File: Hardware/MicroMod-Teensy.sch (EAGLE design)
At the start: 73 parts, among them J1 MICROMOD-2222, Q1 20V/4.2A/52mΩ/1.4W, Q2 20V/0.2A/8MHz/1.2Ω/1Vth, U1 IMXRT1062DV10X10, U3 MKL02Z32VFG4, U4 W25QXX128MBIT-6X5, Y1 32.768kHz, Y2 24MHz

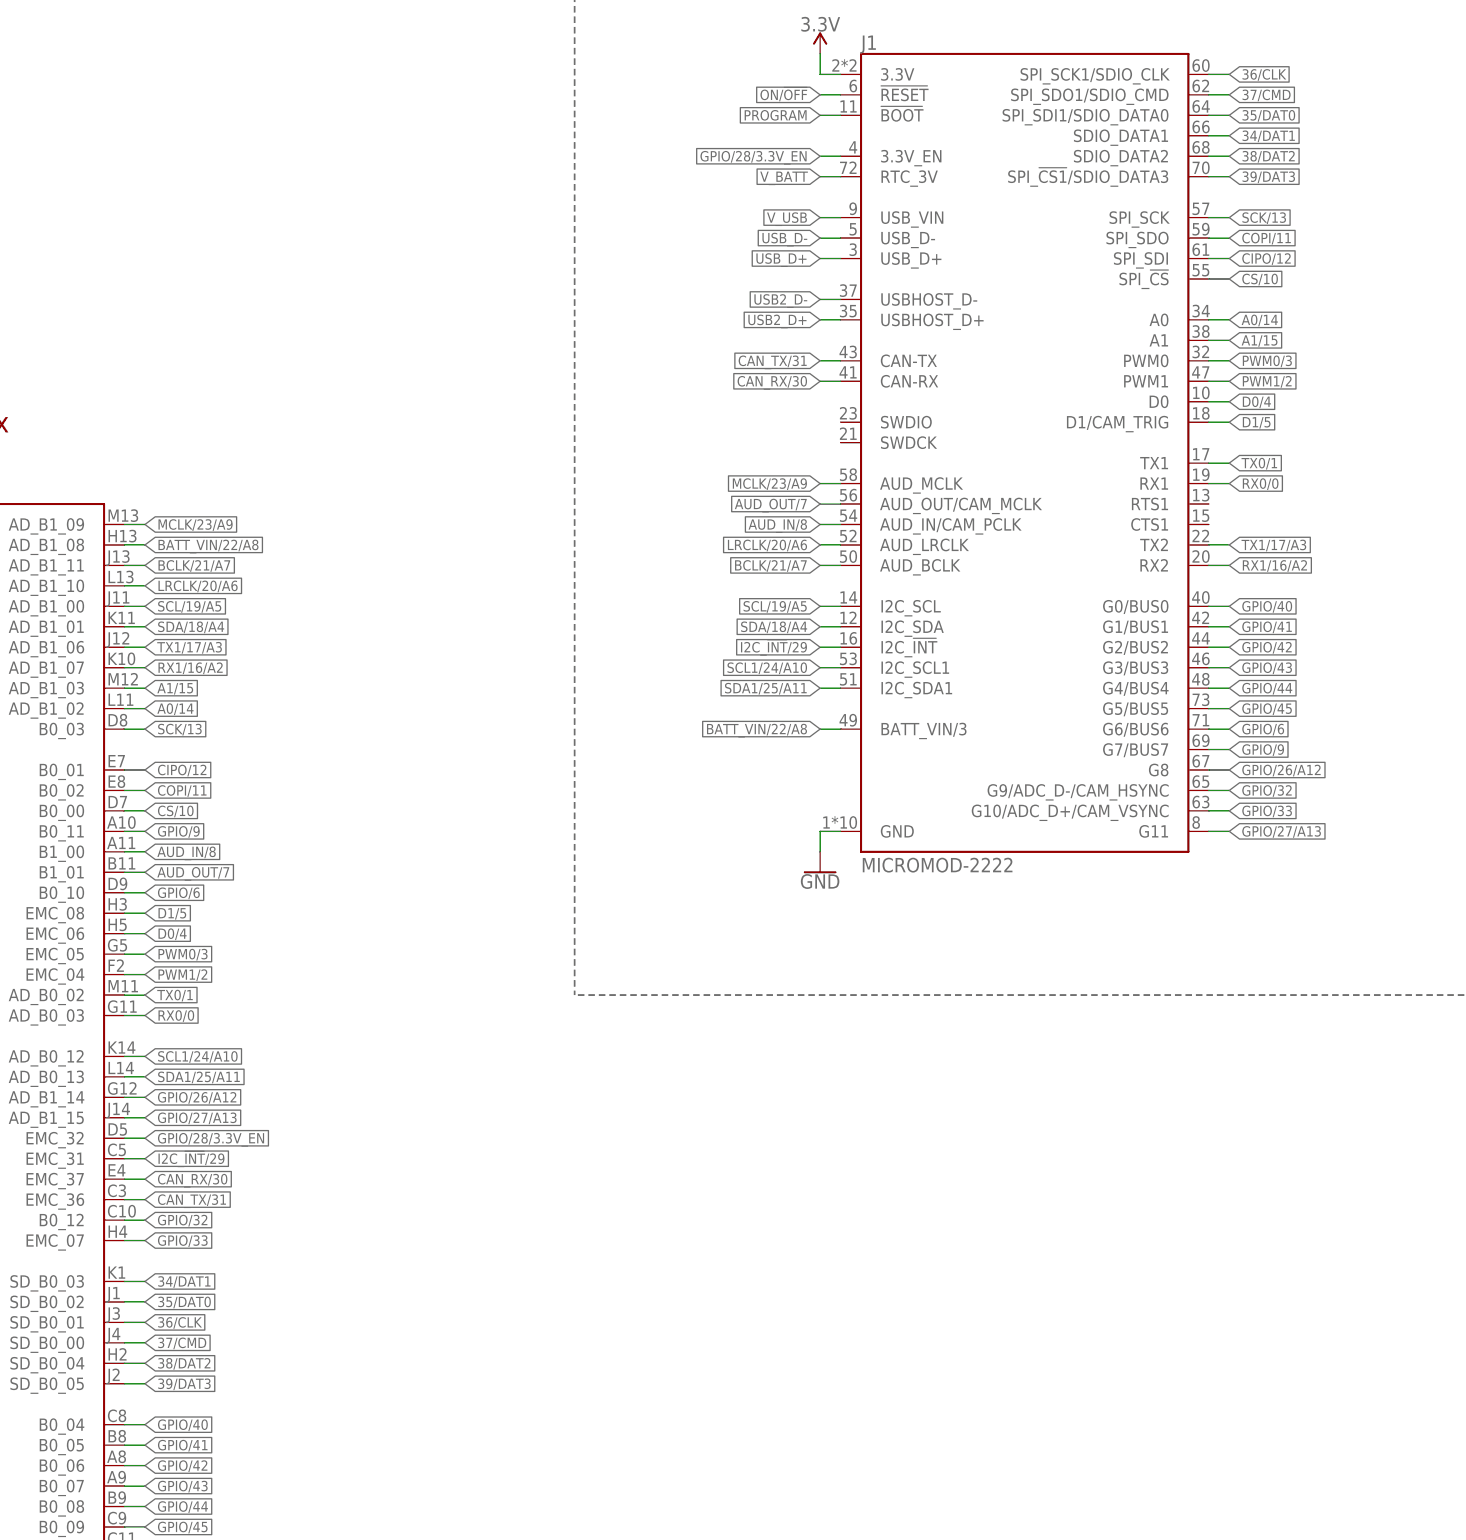
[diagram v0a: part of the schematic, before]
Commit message: Correct swapped pin numbers on DAT2/3.
This stems from an error in the original Teensy 4.0 schematic. It was found and corrected but Paul swapped the pin numbers where we swapped the net names. This should get us back on the same page.
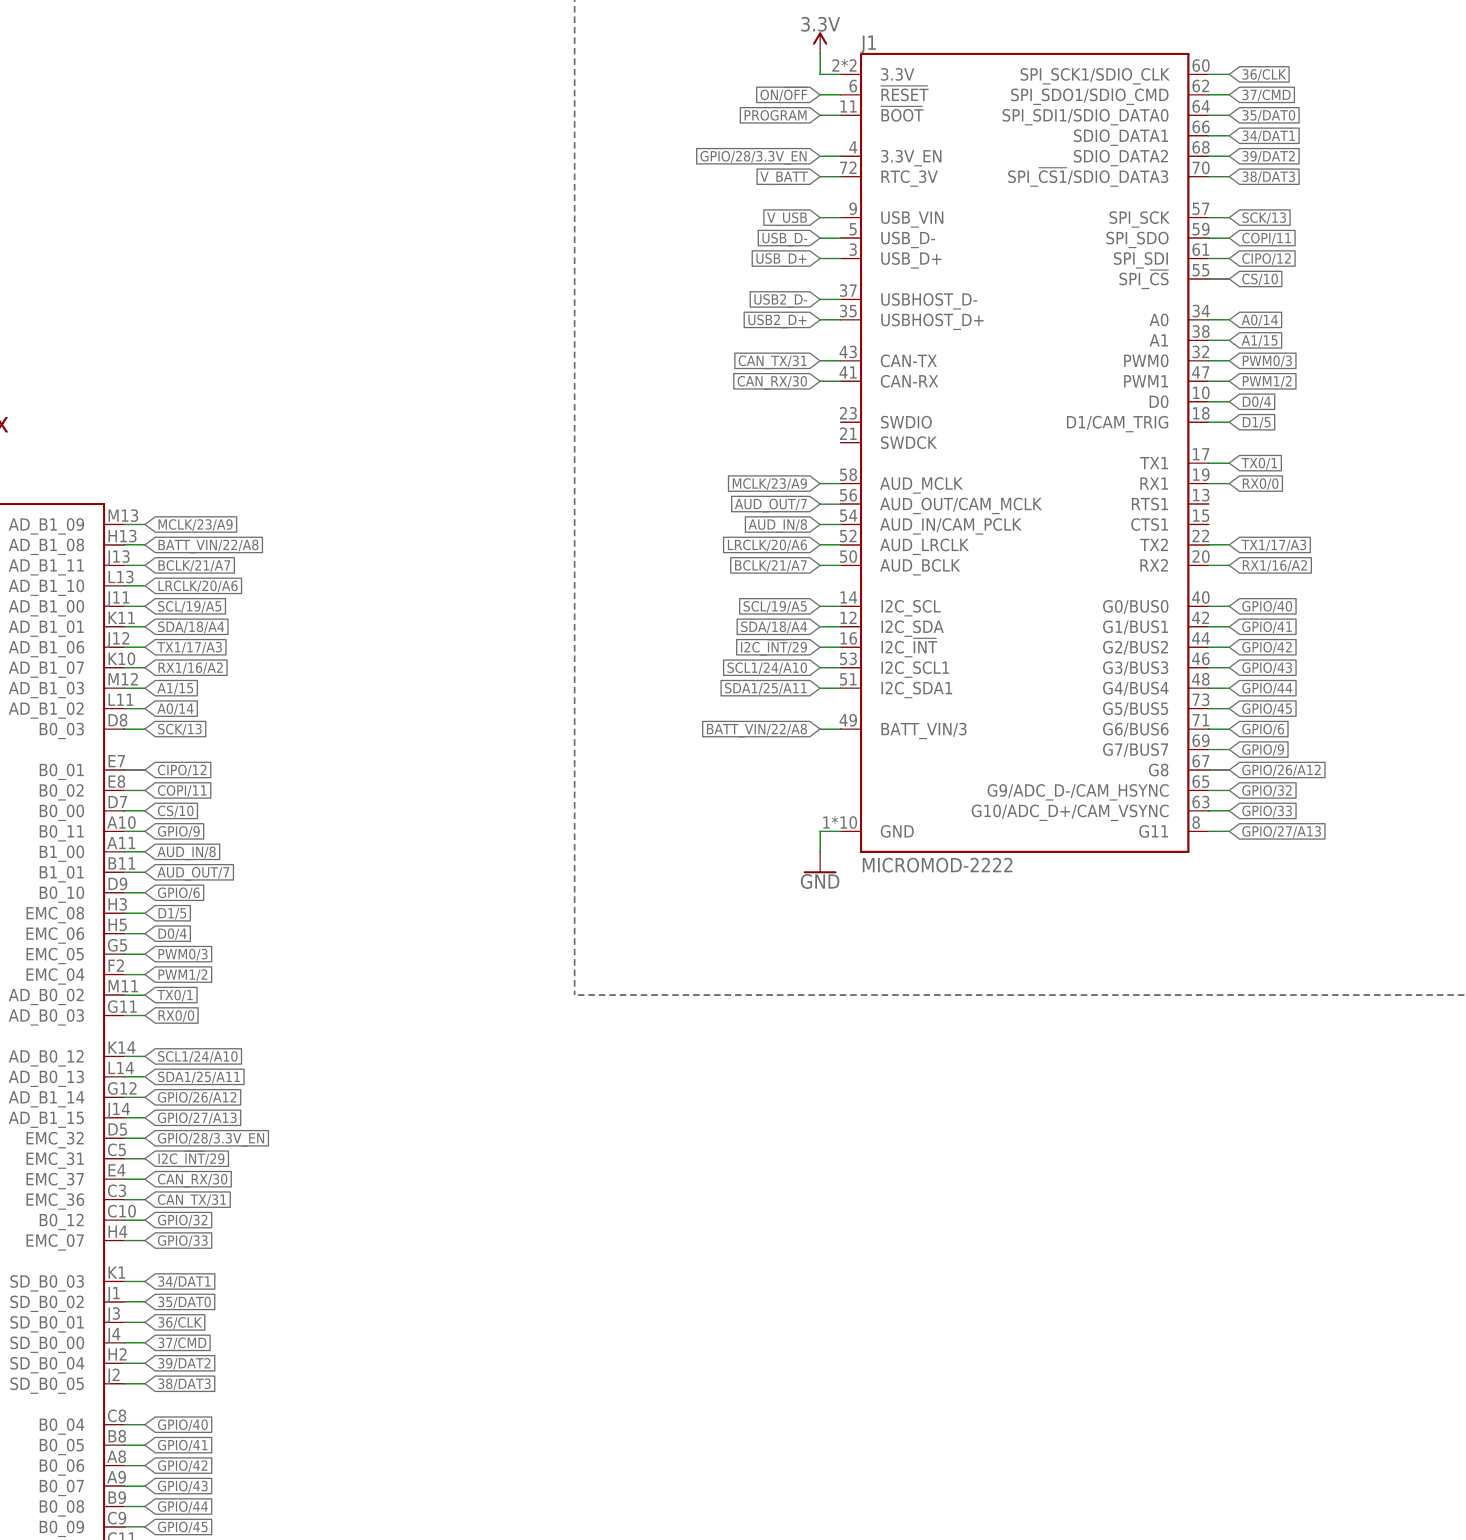
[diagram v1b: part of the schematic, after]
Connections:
- net 38/DAT2 renamed 39/DAT2
- net 39/DAT3 renamed 38/DAT3
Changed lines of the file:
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@@
 <?xml version="1.0" encoding="utf-8"?>
 <!DOCTYPE eagle SYSTEM "eagle.dtd">
-<eagle version="9.6.0">
+<eagle version="9.6.2">
 <drawing>
 <settings>
@@
 </segment>
 </net>
-<net name="39/DAT3" class="0">
+<net name="38/DAT3" class="0">
 <segment>
 <wire x1="297.18" y1="241.3" x2="299.72" y2="241.3" width="0.1524" layer="91"/>
@@
 </segment>
 </net>
-<net name="38/DAT2" class="0">
+<net name="39/DAT2" class="0">
 <segment>
 <wire x1="162.56" y1="93.98" x2="165.1" y2="93.98" width="0.1524" layer="91"/>

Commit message: Revert "Correct swapped pin numbers on DAT2/3."
This reverts commit 18efc8621dbd46baebb258ee20b759296ca70ac1.

Pin swap was fixed in software: https://github.com/PaulStoffregen/cores/commit/17f652645c1af3bb0190d6b3769d48358c7ad276
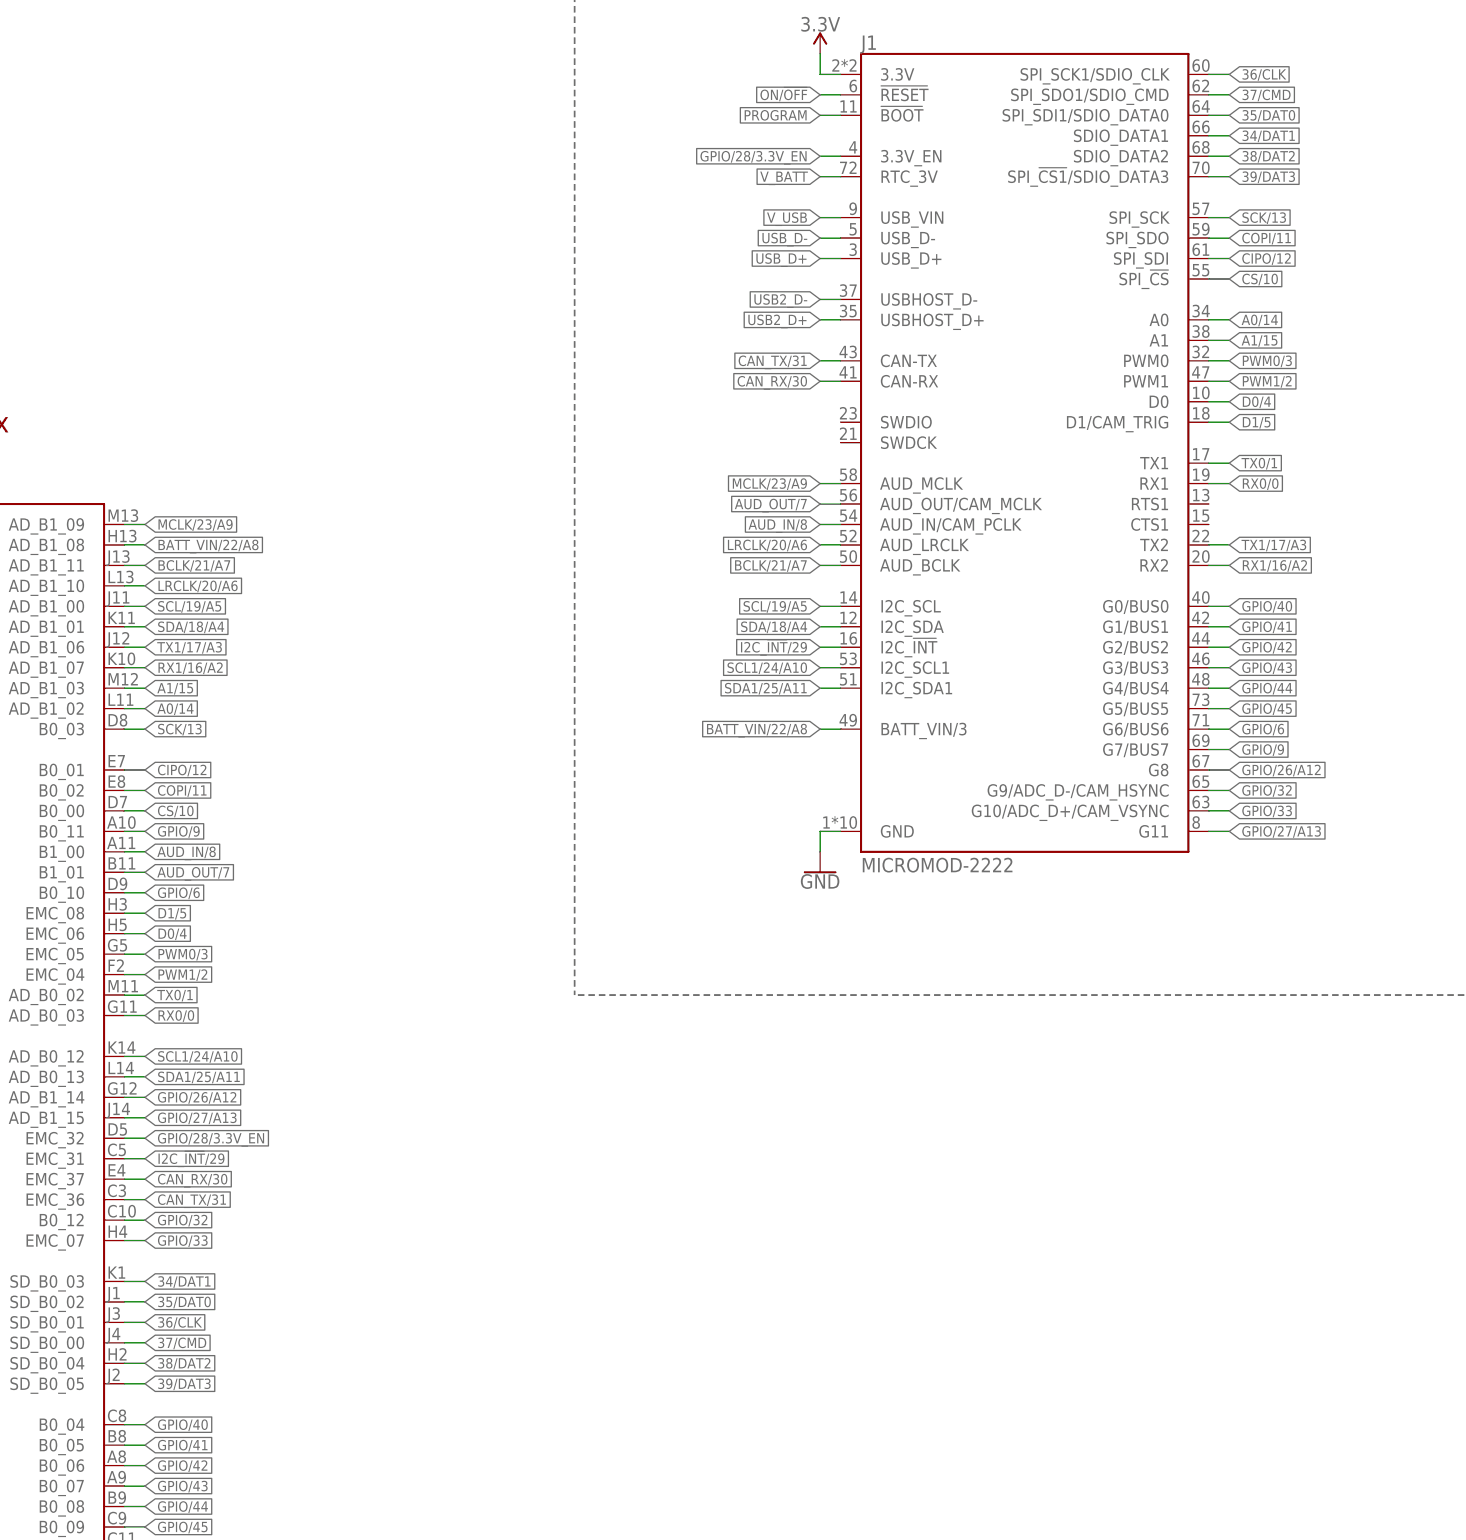
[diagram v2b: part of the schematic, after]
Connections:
- net 38/DAT3 renamed 39/DAT3
- net 39/DAT2 renamed 38/DAT2
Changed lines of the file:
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@@
 <?xml version="1.0" encoding="utf-8"?>
 <!DOCTYPE eagle SYSTEM "eagle.dtd">
-<eagle version="9.6.2">
+<eagle version="9.6.0">
 <drawing>
 <settings>
@@
 </segment>
 </net>
-<net name="38/DAT3" class="0">
+<net name="39/DAT3" class="0">
 <segment>
 <wire x1="297.18" y1="241.3" x2="299.72" y2="241.3" width="0.1524" layer="91"/>
@@
 </segment>
 </net>
-<net name="39/DAT2" class="0">
+<net name="38/DAT2" class="0">
 <segment>
 <wire x1="162.56" y1="93.98" x2="165.1" y2="93.98" width="0.1524" layer="91"/>
